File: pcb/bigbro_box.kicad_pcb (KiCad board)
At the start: 2 copper layers, 100 x 58 mm, 56 parts, among them J1 Current Sense, J2 Display, J3 Mains, J4 Debug, J5 RFID, J6 Relay, J7 Ext, K1 G5LE-1, Q1 MMBT3904, Q2 MMBT3904, Q3 BSS138, Q4 MMBT3906, Q5 MMBT3904, SW1 Card switch, SW2 SW_SPST, SW3 SW_SPST, U1 ESP32-WROOM-32, U2 AP1117-33, U3 4011, U4 4011, U5 RDM6300

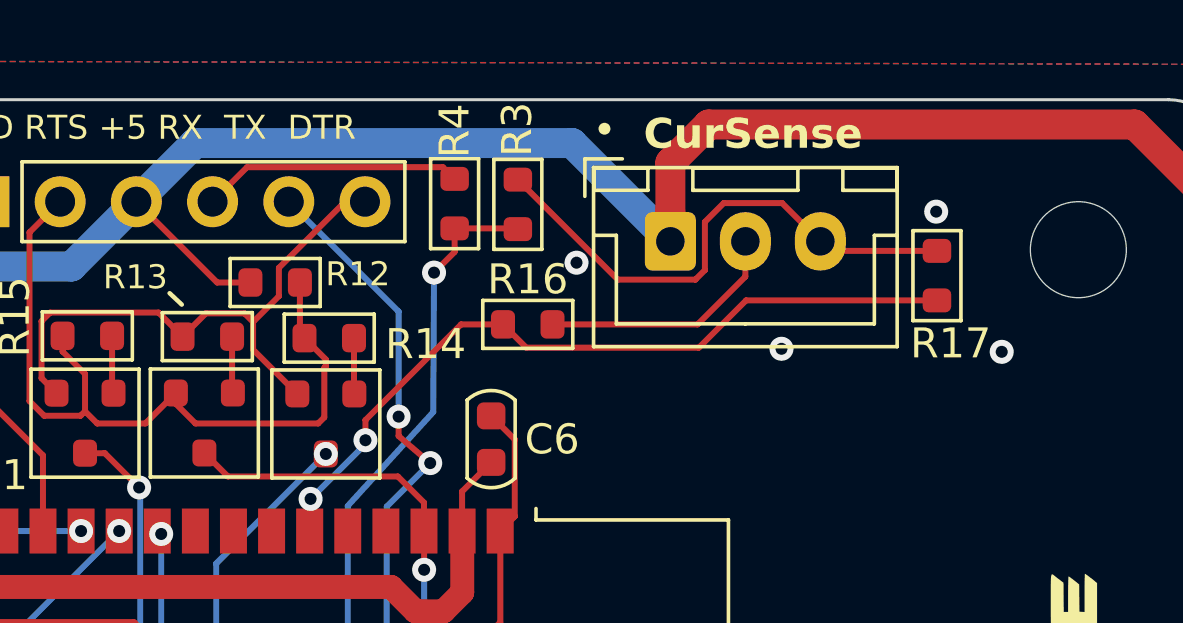
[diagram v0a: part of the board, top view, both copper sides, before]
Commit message: Use zener.
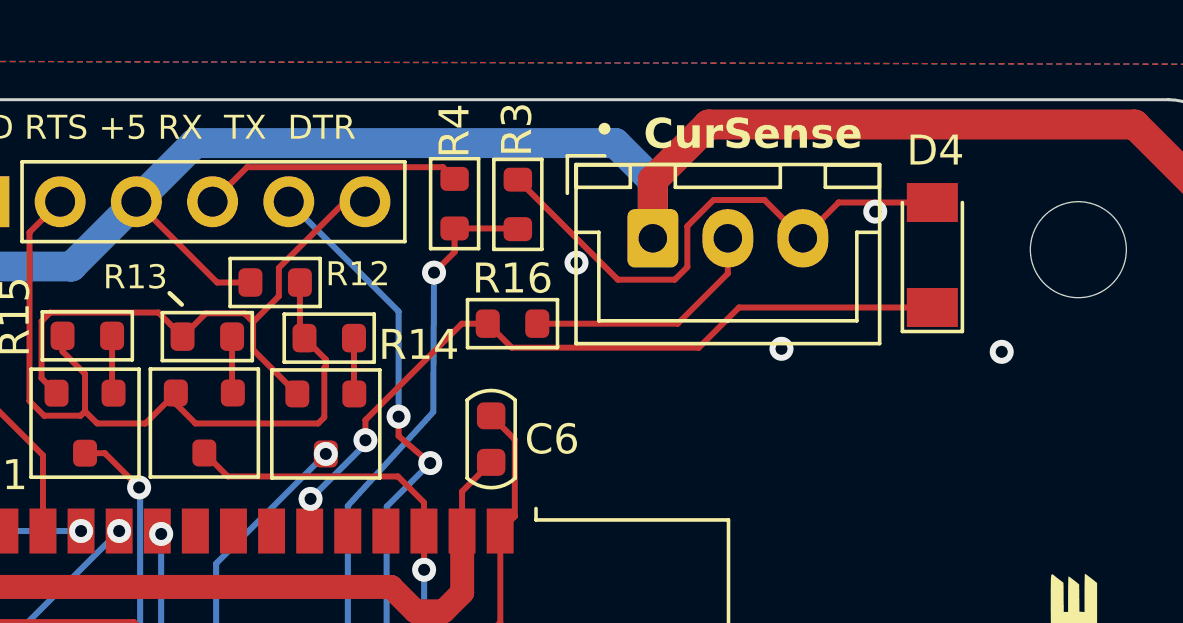
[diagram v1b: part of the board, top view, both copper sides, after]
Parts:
- removed R17: 2k2, PCM_Resistor_SMD_AKL:R_0603_1608Metric
- added D4: 3V0, Diode_SMD:D_MiniMELF, F.Cu at (156.1, 62.2)
- R16: value 1k2 -> 1k
- moved J1 0.59 mm to (146.8, 61.6)
- moved R16 0.51 mm to (142.1, 64.5)
